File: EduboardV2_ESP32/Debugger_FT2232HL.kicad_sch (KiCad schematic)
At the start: 30 parts, among them U2 FT2232HL, U3 93CxxC, Y1 12MHz

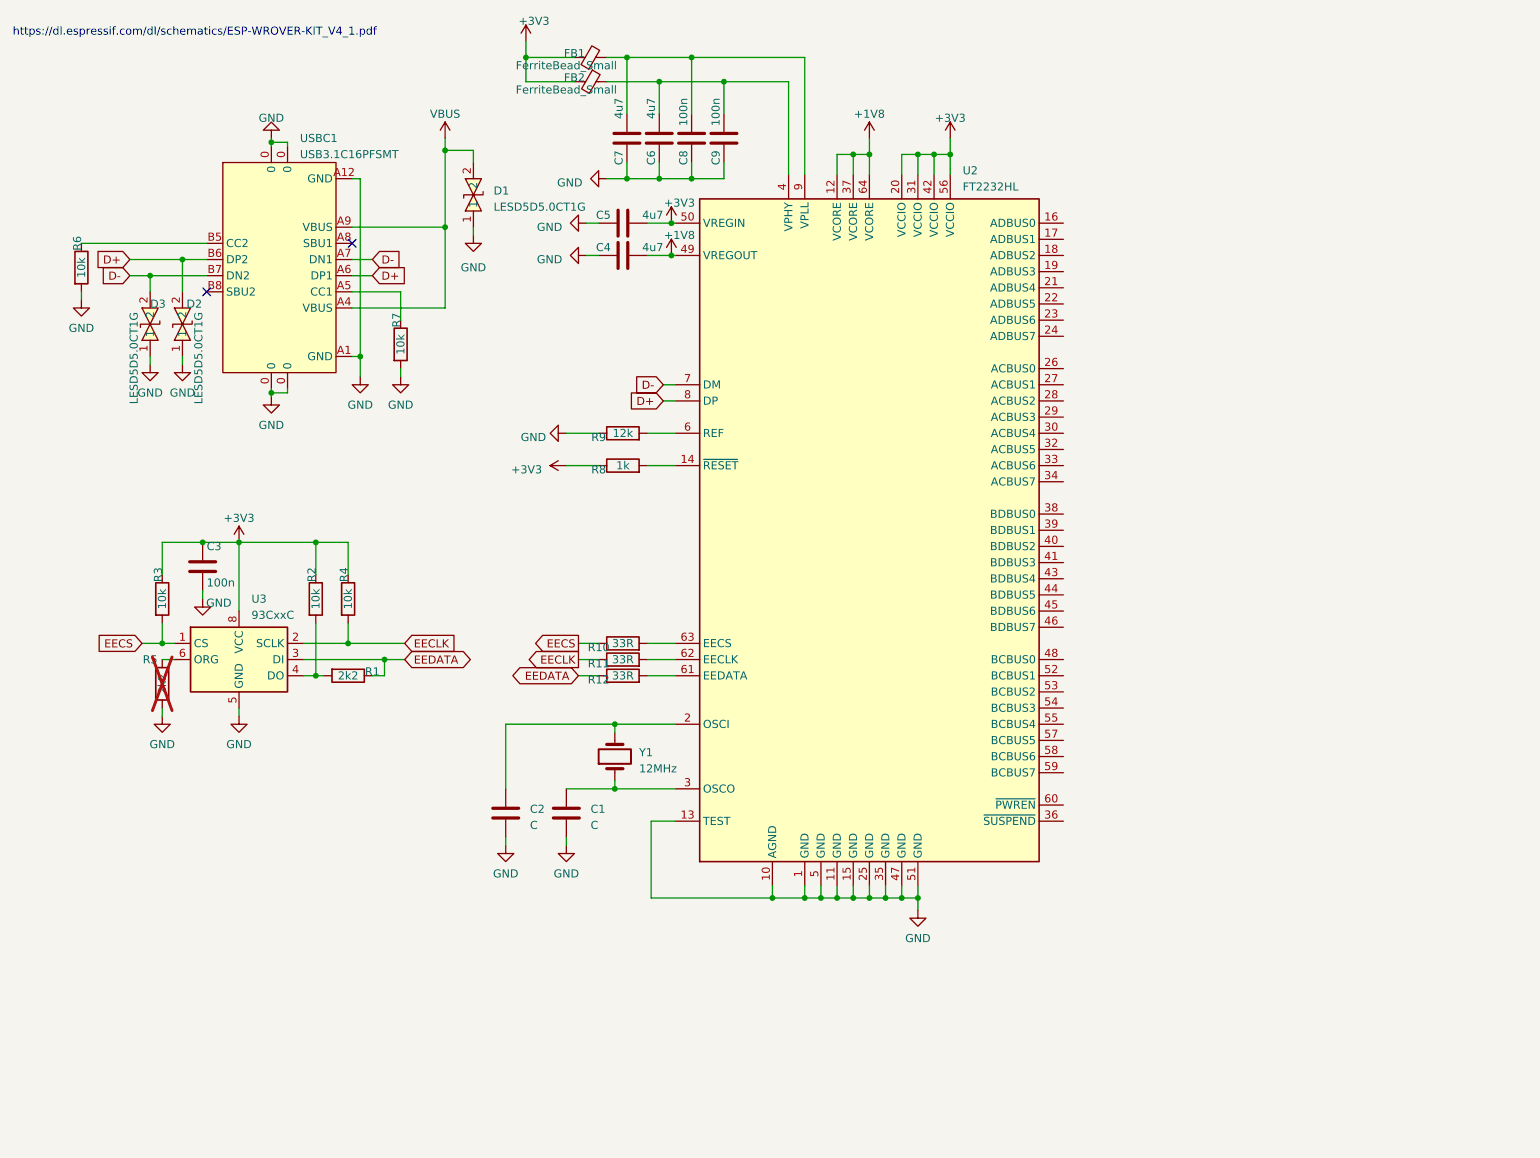
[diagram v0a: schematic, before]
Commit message: work on debug chip
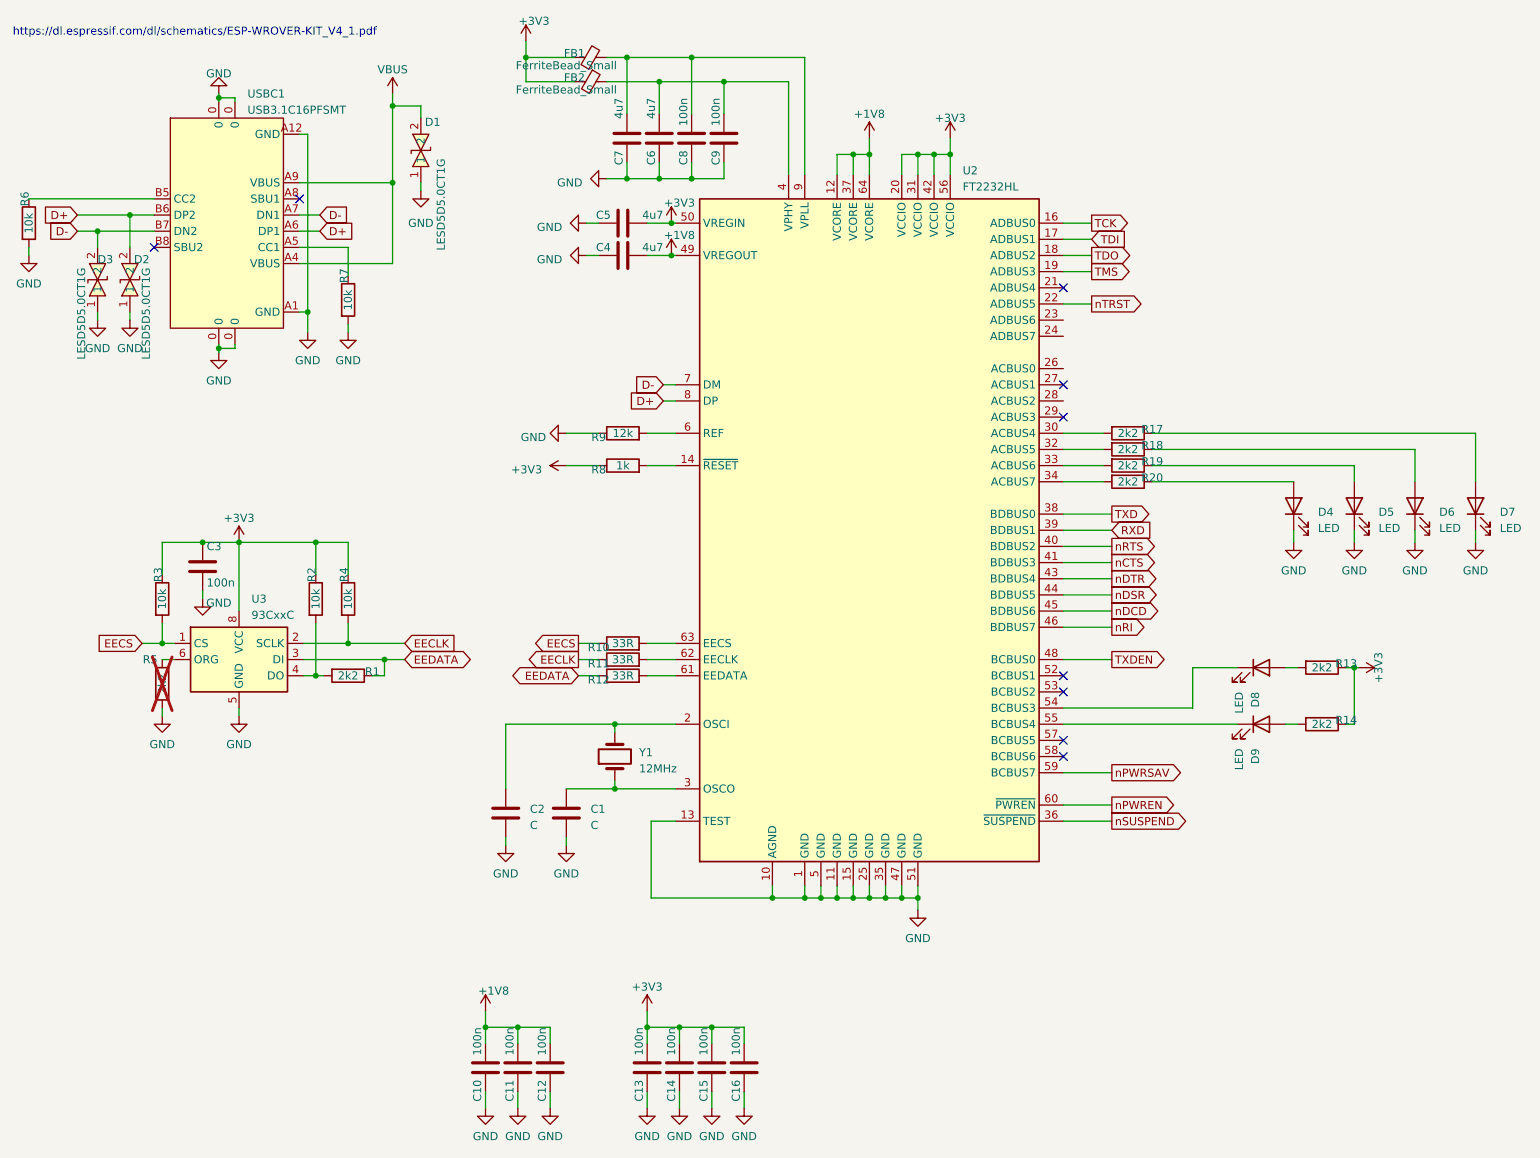
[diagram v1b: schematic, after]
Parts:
- added C10, C11, C12, C13, C14, C15, C16: 100n, symbol Device:C
- added D4, D5, D6, D7, D8, D9: LED, symbol Device:LED
- added R13, R14, R17, R18, R19, R20: 2k2, symbol Device:R
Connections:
- net +1V8: now also C10.2, C11.2, C12.2
- net +3V3: now also C13.2, C14.2, C15.2, C16.2, R13.1, R14.1
- net GND: now also C10.1, C11.1, C12.1, C13.1, C14.1, C15.1, C16.1, D4.1 (K), D5.1 (K), D6.1 (K), D7.1 (K)
- net TCK: now reaches U2.16 (ADBUS0)
- net TDI: now reaches U2.17 (ADBUS1)
- net TDO: now reaches U2.18 (ADBUS2)
- net TMS: now reaches U2.19 (ADBUS3)
- net nTRST: now reaches U2.22 (ADBUS5)
- net at U2.30 (ACBUS4): now also R17.2
- net at U2.32 (ACBUS5): now also R18.2
- net at U2.33 (ACBUS6): now also R19.2
- net at U2.34 (ACBUS7): now also R20.2
- net nSUSPEND: now reaches U2.36 (~{SUSPEND})
- net TXD: now reaches U2.38 (BDBUS0)
- net RXD: now reaches U2.39 (BDBUS1)
- net nRTS: now reaches U2.40 (BDBUS2)
- net nCTS: now reaches U2.41 (BDBUS3)
- net nDTR: now reaches U2.43 (BDBUS4)
- net nDSR: now reaches U2.44 (BDBUS5)
- net nDCD: now reaches U2.45 (BDBUS6)
- net nRI: now reaches U2.46 (BDBUS7)
- net TXDEN: now reaches U2.48 (BCBUS0)
- net at U2.54 (BCBUS3): now also D8.1 (K)
- net at U2.55 (BCBUS4): now also D9.1 (K)
- net nPWRSAV: now reaches U2.59 (BCBUS7)
- net nPWREN: now reaches U2.60 (~{PWREN})
- new net: D9.2 (A), R14.2
- new net: D4.2 (A), R20.1
- new net: D8.2 (A), R13.2
- new net: D6.2 (A), R18.1
- new net: D5.2 (A), R19.1
- new net: D7.2 (A), R17.1
- no-connect marks 2 -> 9
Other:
- moved on the sheet: D1, D2, D3, R6, R7, USBC1
